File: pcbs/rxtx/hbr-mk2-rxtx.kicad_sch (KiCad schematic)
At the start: 53 parts, among them J1 Conn_01x02, J2 Conn_01x02, J3 Conn_01x02, J4 Conn_01x02, J5 Conn_01x02, K1 G6K-2F-Y, K2 G6K-2F-Y, K3 G6K-2F-Y, K4 G6K-2F-Y, K5 G6K-2F-Y, K6 G6K-2F-Y, Y1 9.000, Y10 9.000, Y11 9.000, Y12 9.000, Y13 9.000, Y14 9.000, Y15 9.000, Y2 9.000, Y3 9.000, Y4 9.000, Y5 9.000, Y6 9.000, Y7 9.000, Y8 9.000, Y9 9.000

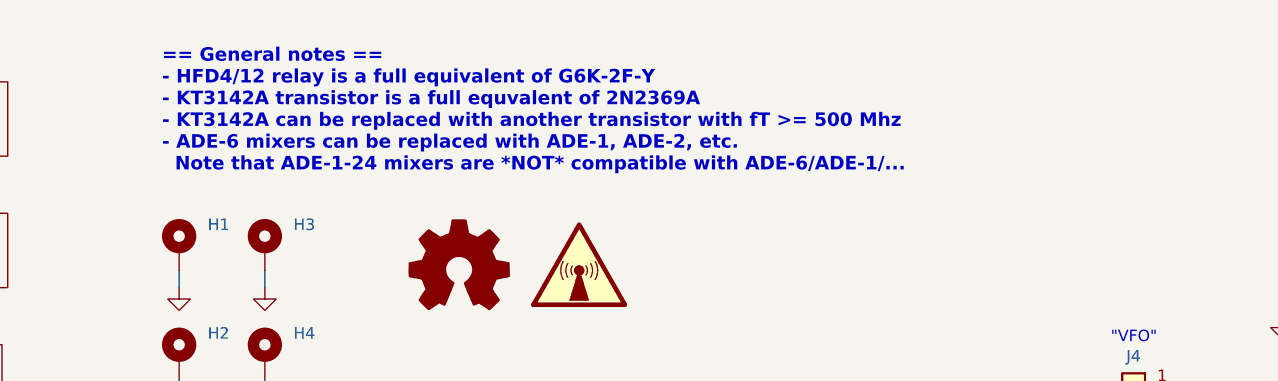
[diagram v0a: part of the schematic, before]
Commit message: Minor changes
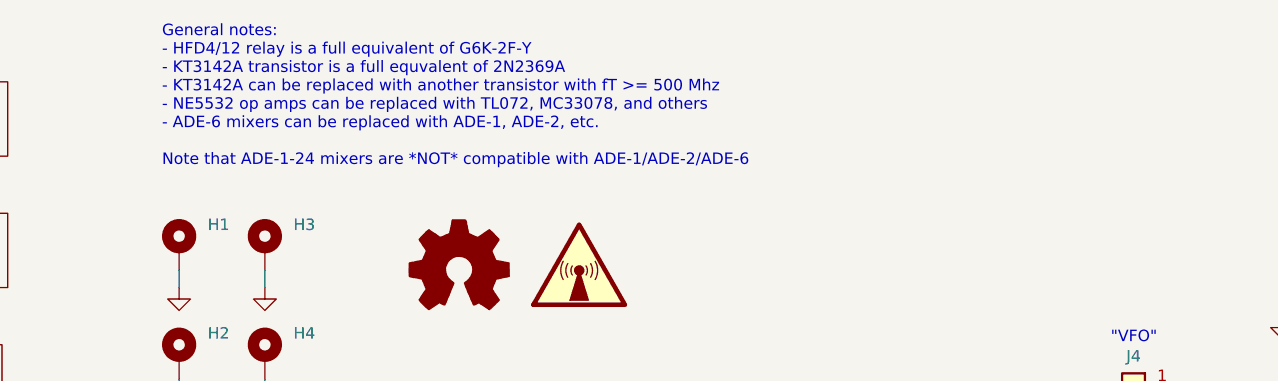
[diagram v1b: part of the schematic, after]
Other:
- note added: "General notes: - HFD4/12 relay is a full equivalent of G6K-2F-Y - KT3142A transistor is a full equvalent of 2N2369A - KT3142A can be replaced with another transistor with fT >= 500 Mhz - NE5532 op amps can be replaced with TL072, MC33078, and others - ADE-6 mixers can be replaced with ADE-1, ADE-2, etc. Note that ADE-1-24 mixers are *NOT* compatible with ADE-1/ADE-2/ADE-6"
- note removed: "== General notes == - HFD4/12 relay is a full equivalent of G6K-2F-Y - KT3142A transistor is a full equvalent of 2N2369A - KT3142A can be replaced with another transistor with fT >= 500 Mhz - ADE-6 mixers can be replaced with ADE-1, ADE-2, etc. Note that ADE-1-24 mixers are *NOT* compatible with ADE-6/ADE-1/..."
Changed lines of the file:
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@@
     (effects (font (size 1.27 1.27)) (justify right bottom))
   )
-  (text "== General notes ==\n- HFD4/12 relay is a full equivalent of G6K-2F-Y\n- KT3142A transistor is a full equvalent of 2N2369A\n- KT3142A can be replaced with another transistor with fT >= 500 Mhz\n- ADE-6 mixers can be replaced with ADE-1, ADE-2, etc.\n  Note that ADE-1-24 mixers are *NOT* compatible with ADE-6/ADE-1/..."
-    (at 55.245 31.115 0)
-    (effects (font (face "Courier New") (size 1.5 1.5) (thickness 0.3) bold) (justify left bottom))
+  (text "General notes:\n- HFD4/12 relay is a full equivalent of G6K-2F-Y\n- KT3142A transistor is a full equvalent of 2N2369A\n- KT3142A can be replaced with another transistor with fT >= 500 Mhz\n- NE5532 op amps can be replaced with TL072, MC33078, and others\n- ADE-6 mixers can be replaced with ADE-1, ADE-2, etc.\n\nNote that ADE-1-24 mixers are *NOT* compatible with ADE-1/ADE-2/ADE-6"
+    (at 55.245 30.48 0)
+    (effects (font (size 1.27 1.27)) (justify left bottom))
   )
   (text "see /RX/" (at 281.94 132.715 0)
